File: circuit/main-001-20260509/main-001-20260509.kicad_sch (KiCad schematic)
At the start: 13 parts, among them Q1 BSS138, Q2 BSS138, U1 DEV-16771

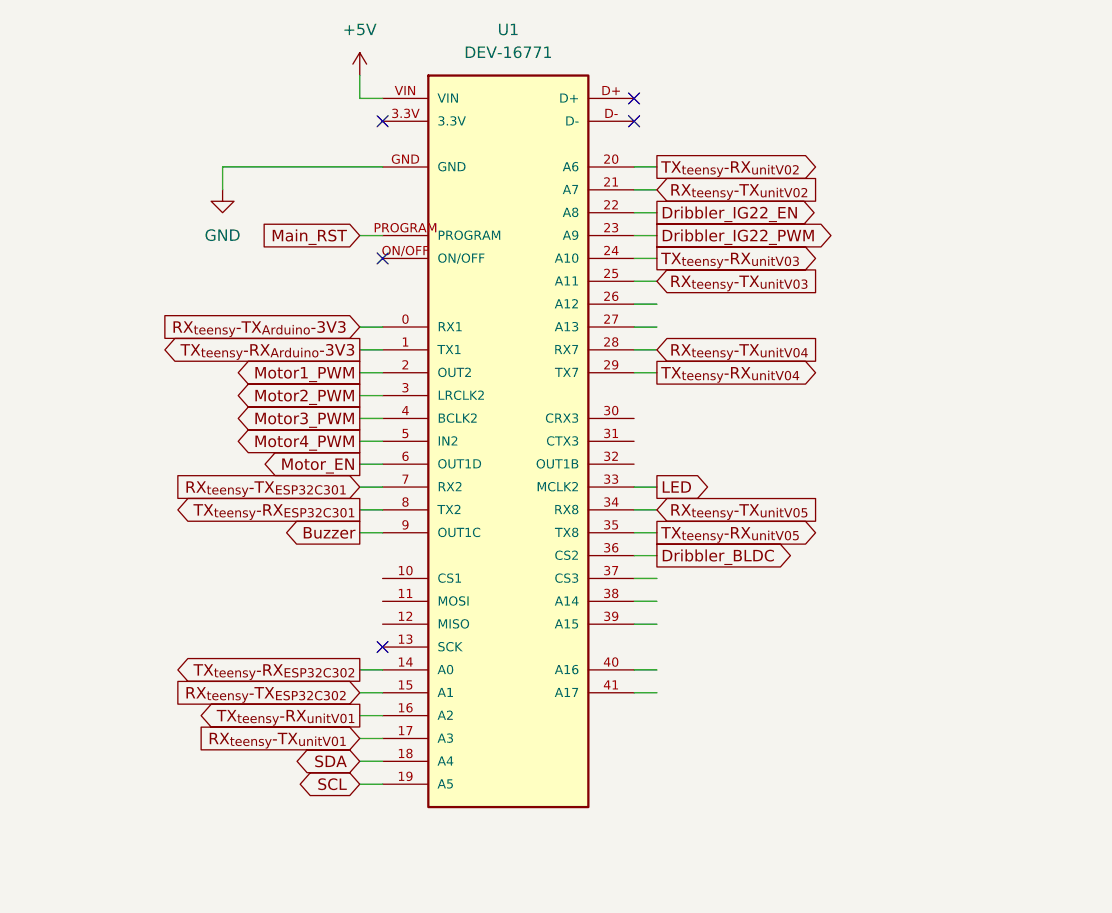
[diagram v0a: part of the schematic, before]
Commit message: Create ネオピクセル基板完成した
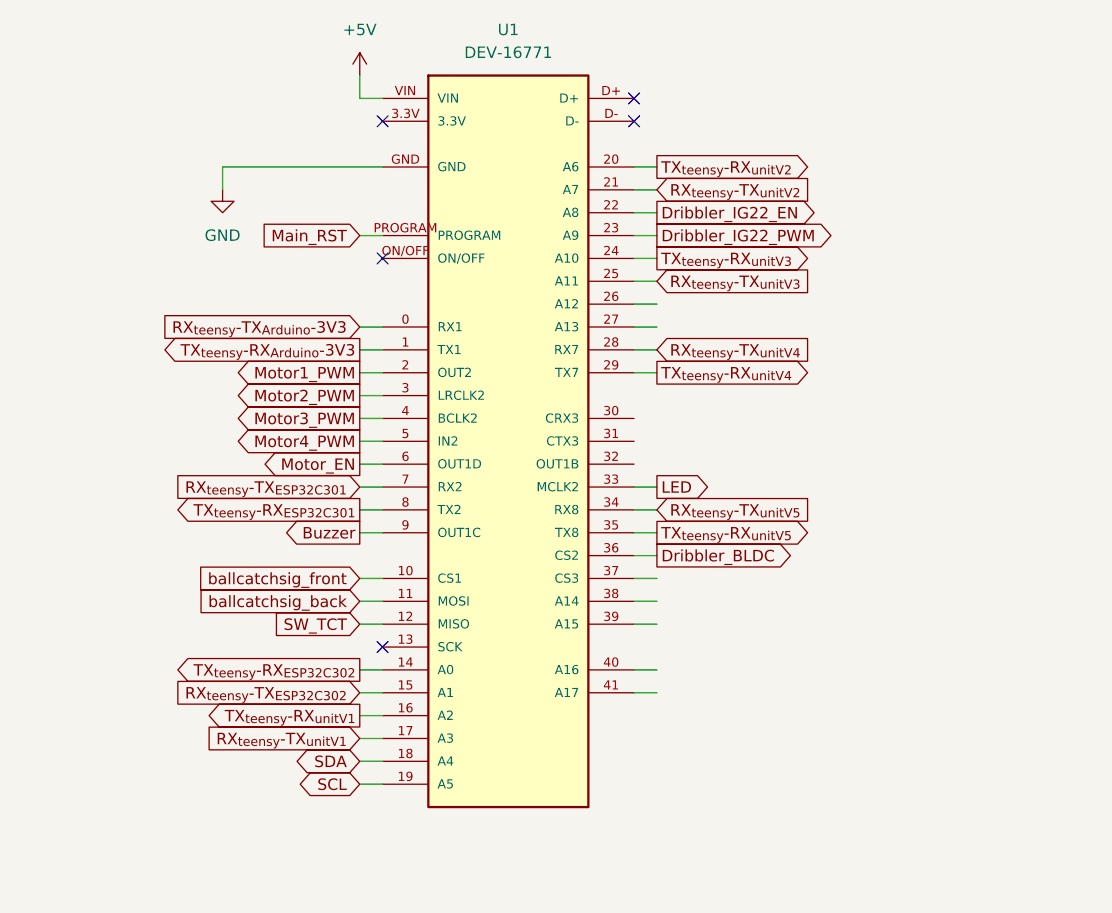
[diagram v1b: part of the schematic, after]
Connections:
- net ballcatchsig_front: now reaches U1.10 (CS1)
- net ballcatchsig_back: now reaches U1.11 (MOSI)
- net SW_TCT: now reaches U1.12 (MISO)
- net RX_{teensy}-TX_{unitV01} renamed RX_{teensy}-TX_{unitV1}
- net RX_{teensy}-TX_{unitV02} renamed RX_{teensy}-TX_{unitV2}
- net RX_{teensy}-TX_{unitV03} renamed RX_{teensy}-TX_{unitV3}
- net RX_{teensy}-TX_{unitV04} renamed RX_{teensy}-TX_{unitV4}
- net RX_{teensy}-TX_{unitV05} renamed RX_{teensy}-TX_{unitV5}
- net TX_{teensy}-RX_{unitV01} renamed TX_{teensy}-RX_{unitV1}
- net TX_{teensy}-RX_{unitV02} renamed TX_{teensy}-RX_{unitV2}
- net TX_{teensy}-RX_{unitV03} renamed TX_{teensy}-RX_{unitV3}
- net TX_{teensy}-RX_{unitV04} renamed TX_{teensy}-RX_{unitV4}
- net TX_{teensy}-RX_{unitV05} renamed TX_{teensy}-RX_{unitV5}
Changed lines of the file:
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@@
+	(wire
+		(pts
+			(xy 38.1 83.82) (xy 40.64 83.82)
+		)
+		(stroke
+			(width 0)
+			(type default)
+		)
+	)
 	(wire
 		(pts
@@
 	(wire
 		(pts
+			(xy 38.1 81.28) (xy 40.64 81.28)
+		)
+		(stroke
+			(width 0)
+			(type default)
+		)
+	)
+	(wire
+		(pts
+			(xy 38.1 86.36) (xy 40.64 86.36)
+		)
+		(stroke
+			(width 0)
+			(type default)
+		)
+	)
+	(wire
+		(pts
 			(xy 52.07 142.24) (xy 52.07 140.97)
 		)
@@
 		)
 	)
-	(global_label "RX_{teensy}-TX_{unitV05}"
+	(global_label "RX_{teensy}-TX_{unitV5}"
 		(shape input)
 		(at 71.12 73.66 0)
@@
 		)
 		(property "Intersheetrefs" "${INTERSHEET_REFS}"
-			(at 90.9321 73.66 0)
+			(at 89.9645 73.66 0)
 			(hide yes)
 			(show_name no)
@@
 		)
 	)
+	(global_label "ballcatchsig_back"
+		(shape input)
+		(at 38.1 83.82 180)
+		(fields_autoplaced yes)
+		(effects
+			(font
+				(size 1.27 1.27)
+			)
+			(justify right)
+		)
+		(property "Intersheetrefs" "${INTERSHEET_REFS}"
+			(at 18.1213 83.82 0)
+			(hide yes)
+			(show_name no)
+			(do_not_autoplace no)
+			(effects
+				(font
+					(size 1.27 1.27)
+				)
+				(justify right)
+			)
+		)
+	)
 	(global_label "Motor3_PWM"
 		(shape output)
@@
 		)
 	)
+	(global_label "ballcatchsig_front"
+		(shape input)
+		(at 38.1 81.28 180)
+		(fields_autoplaced yes)
+		(effects
+			(font
+				(size 1.27 1.27)
+			)
+			(justify right)
+		)
+		(property "Intersheetrefs" "${INTERSHEET_REFS}"
+			(at 18.0004 81.28 0)
+			(hide yes)
+			(show_name no)
+			(do_not_autoplace no)
+			(effects
+				(font
+					(size 1.27 1.27)
+				)
+				(justify right)
+			)
+		)
+	)
 	(global_label "RX_{teensy}-TX_{ESP32C301}"
 		(shape input)
@@
 		)
 	)
-	(global_label "RX_{teensy}-TX_{unitV02}"
+	(global_label "RX_{teensy}-TX_{unitV2}"
 		(shape input)
 		(at 71.12 38.1 0)
@@
 		)
 		(property "Intersheetrefs" "${INTERSHEET_REFS}"
-			(at 90.9321 38.1 0)
+			(at 89.9645 38.1 0)
 			(hide yes)
 			(show_name no)
@@
 		)
 	)
-	(global_label "RX_{teensy}-TX_{unitV03}"
+	(global_label "RX_{teensy}-TX_{unitV3}"
 		(shape input)
 		(at 71.12 48.26 0)
@@
 		)
 		(property "Intersheetrefs" "${INTERSHEET_REFS}"
-			(at 90.9321 48.26 0)
+			(at 89.9645 48.26 0)
 			(hide yes)
 			(show_name no)
@@
 		)
 	)
-	(global_label "RX_{teensy}-TX_{unitV01}"
+	(global_label "RX_{teensy}-TX_{unitV1}"
 		(shape input)
 		(at 38.1 99.06 180)
@@
 		)
 		(property "Intersheetrefs" "${INTERSHEET_REFS}"
-			(at 18.2879 99.06 0)
+			(at 19.2555 99.06 0)
 			(hide yes)
 			(show_name no)
@@
 		)
 	)
-	(global_label "RX_{teensy}-TX_{unitV04}"
+	(global_label "RX_{teensy}-TX_{unitV4}"
 		(shape input)
 		(at 71.12 55.88 0)
@@
 		)
 		(property "Intersheetrefs" "${INTERSHEET_REFS}"
-			(at 90.9321 55.88 0)
+			(at 89.9645 55.88 0)
 			(hide yes)
 			(show_name no)
@@
 		)
 	)
-	(global_label "TX_{teensy}-RX_{unitV05}"
+	(global_label "TX_{teensy}-RX_{unitV5}"
 		(shape output)
 		(at 71.12 76.2 0)
@@
 		)
 		(property "Intersheetrefs" "${INTERSHEET_REFS}"
-			(at 90.9321 76.2 0)
+			(at 89.9645 76.2 0)
 			(hide yes)
 			(show_name no)
@@
 		)
 	)
-	(global_label "TX_{teensy}-RX_{unitV01}"
+	(global_label "TX_{teensy}-RX_{unitV1}"
 		(shape output)
 		(at 38.1 96.52 180)
@@
 		)
 		(property "Intersheetrefs" "${INTERSHEET_REFS}"
-			(at 18.2879 96.52 0)
+			(at 19.2555 96.52 0)
 			(hide yes)
 			(show_name no)
@@
 		)
 	)
-	(global_label "TX_{teensy}-RX_{unitV04}"
+	(global_label "TX_{teensy}-RX_{unitV4}"
 		(shape output)
 		(at 71.12 58.42 0)
@@
 		)
 		(property "Intersheetrefs" "${INTERSHEET_REFS}"
-			(at 90.9321 58.42 0)
+			(at 89.9645 58.42 0)
 			(hide yes)
 			(show_name no)
@@
 		)
 	)
-	(global_label "TX_{teensy}-RX_{unitV03}"
+	(global_label "TX_{teensy}-RX_{unitV3}"
 		(shape output)
 		(at 71.12 45.72 0)
@@
 		)
 		(property "Intersheetrefs" "${INTERSHEET_REFS}"
-			(at 90.9321 45.72 0)
+			(at 89.9645 45.72 0)
 			(hide yes)
 			(show_name no)
@@
 		)
 	)
-	(global_label "TX_{teensy}-RX_{unitV02}"
+	(global_label "TX_{teensy}-RX_{unitV2}"
 		(shape output)
 		(at 71.12 35.56 0)
@@
 		)
 		(property "Intersheetrefs" "${INTERSHEET_REFS}"
-			(at 90.9321 35.56 0)
+			(at 89.9645 35.56 0)
 			(hide yes)
 			(show_name no)
@@
 			(hide yes)
 			(show_name no)
+			(do_not_autoplace no)
+			(effects
+				(font
+					(size 1.27 1.27)
+				)
+				(justify right)
+			)
+		)
+	)
+	(global_label "SW_TCT"
+		(shape input)
+		(at 38.1 86.36 180)
+		(fields_autoplaced yes)
+		(effects
+			(font
+				(size 1.27 1.27)
+			)
+			(justify right)
+		)
+		(property "Intersheetrefs" "${INTERSHEET_REFS}"
+			(at 28.2811 86.36 0)
+			(hide yes)
+			(show_name no)
